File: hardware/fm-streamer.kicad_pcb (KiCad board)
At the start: 2 copper layers, 40 x 60 mm, 59 parts, among them J1 USB_A, U1 ESP32_DevKit_V1_DOIT, U2 PCM1772PWR, U3 SI4721

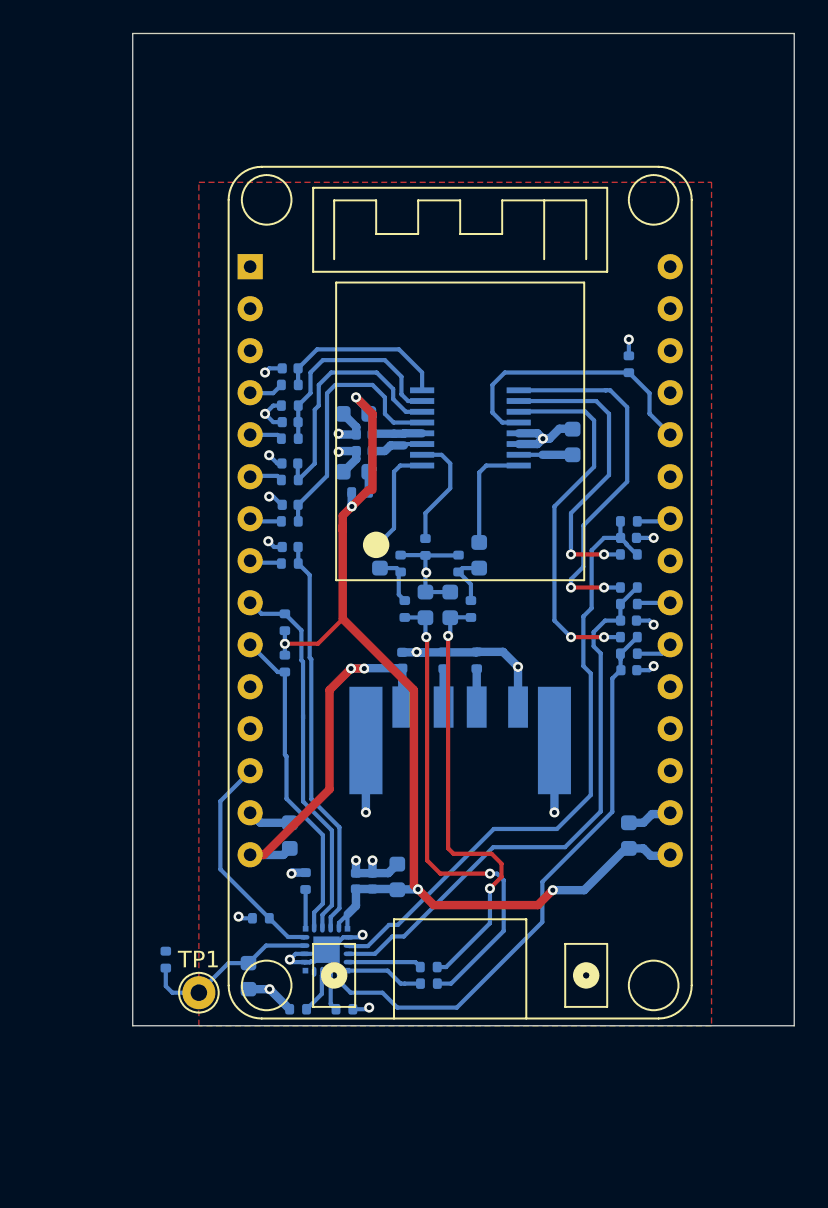
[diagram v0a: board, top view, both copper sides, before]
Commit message: ready for fab quote
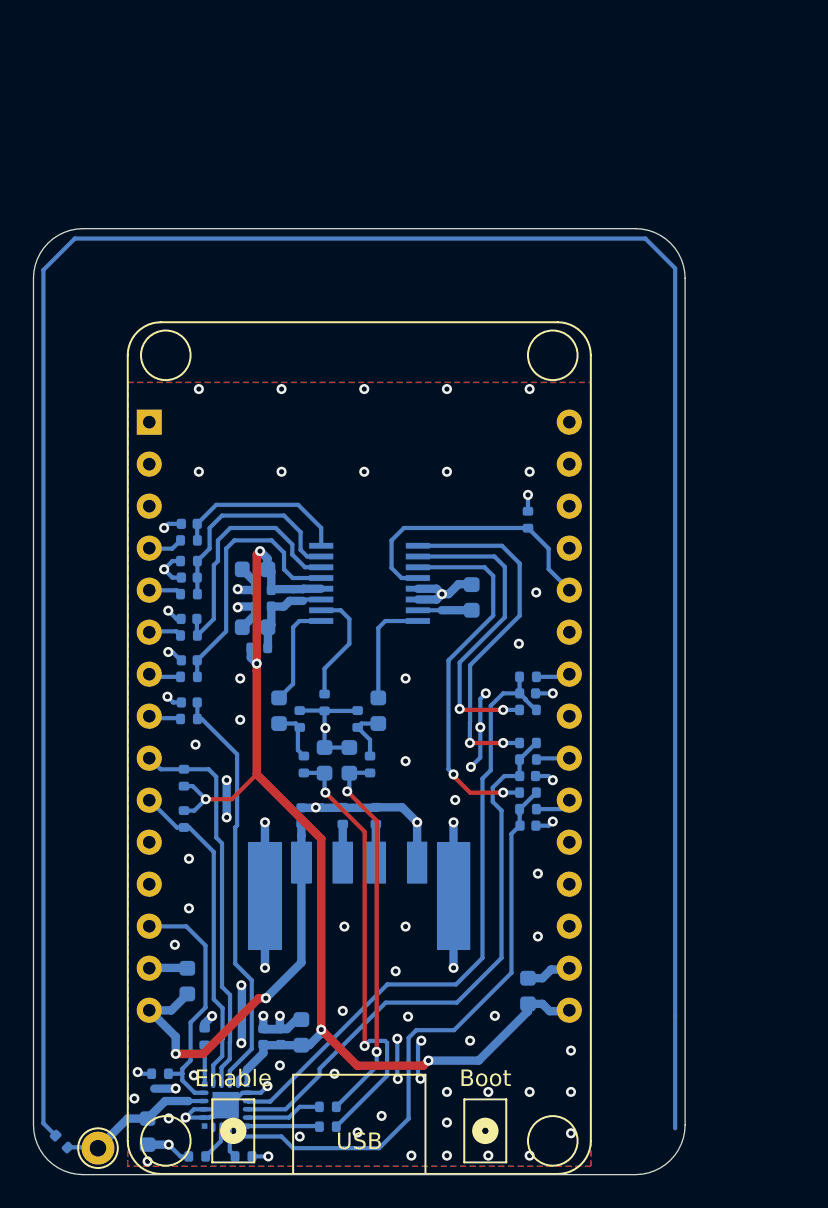
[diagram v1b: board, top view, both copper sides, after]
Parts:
- added J1 (x2): USB_A, Connector_USB:USB_A_Plug_Molex_0480371000_90_deg_mount, B.Cu at (129.7, 102.4)
- moved R14 12.7 mm to (111.7, 118.0), turned to 135 degrees
- moved J1 11.2 mm to (129.7, 102.4)
- moved U1 11.2 mm to (129.7, 74.5)
- moved R12 11.2 mm to (119.1, 98.5)
- moved R19 11.2 mm to (120.3, 111.7)
- moved R3 11.2 mm to (119.1, 96.0)
- moved R1 11.2 mm to (130.7, 98.3)
- moved R2 11.2 mm to (128.7, 98.3)
- moved C10 11.2 mm to (119.4, 86.4)
- moved C11 11.2 mm to (119.4, 83.9)
- moved C12 11.2 mm to (123.4, 86.9)
- moved C13 11.2 mm to (123.9, 85.7)
- moved C14 11.2 mm to (123.4, 83.4)
- moved C15 11.2 mm to (123.9, 84.7)
- moved C19 11.2 mm to (130.8, 92.0)
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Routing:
- net /ANTENNA: track 0.00 -> 144.4 mm
- net GND: track 70.8 -> 97.5 mm, vias 25 -> 89
- net AUDIO_R: track 27.4 -> 23.7 mm
- net AUDIO_L: track 29.5 -> 26.6 mm
- net RADIO_~RST~: track 13.5 -> 15.0 mm
- net +5V: track 22.8 -> 24.3 mm
- net Net-(L1-Pad1): track 10.8 -> 9.43 mm
- net RADIO_REFCLK: track 24.3 -> 25.2 mm
- net I2S_DCLK: track 35.3 -> 36.2 mm
- net Net-(R29-Pad1): track 18.2 -> 18.9 mm
- net I2C_SDA: track 22.9 -> 23.6 mm
- net Net-(R30-Pad1): track 22.3 -> 21.7 mm
- added copper zone on B.Cu, net GND
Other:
- board size 40 x 60 mm -> 39.4 x 57.2 mm
- board text added: "ANT"
- board text added: "FM STREAMER REV0"
